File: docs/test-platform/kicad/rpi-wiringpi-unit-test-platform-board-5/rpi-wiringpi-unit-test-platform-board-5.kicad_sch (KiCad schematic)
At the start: 14 parts, among them J1 JST_IN_PWR, J2 JST_IN_SIG, J3 JST_IN_LCD, J4 JST_OUT_ARDUINO, M1 Logic_Converter_4_Pin, SW1 SW_CTRL

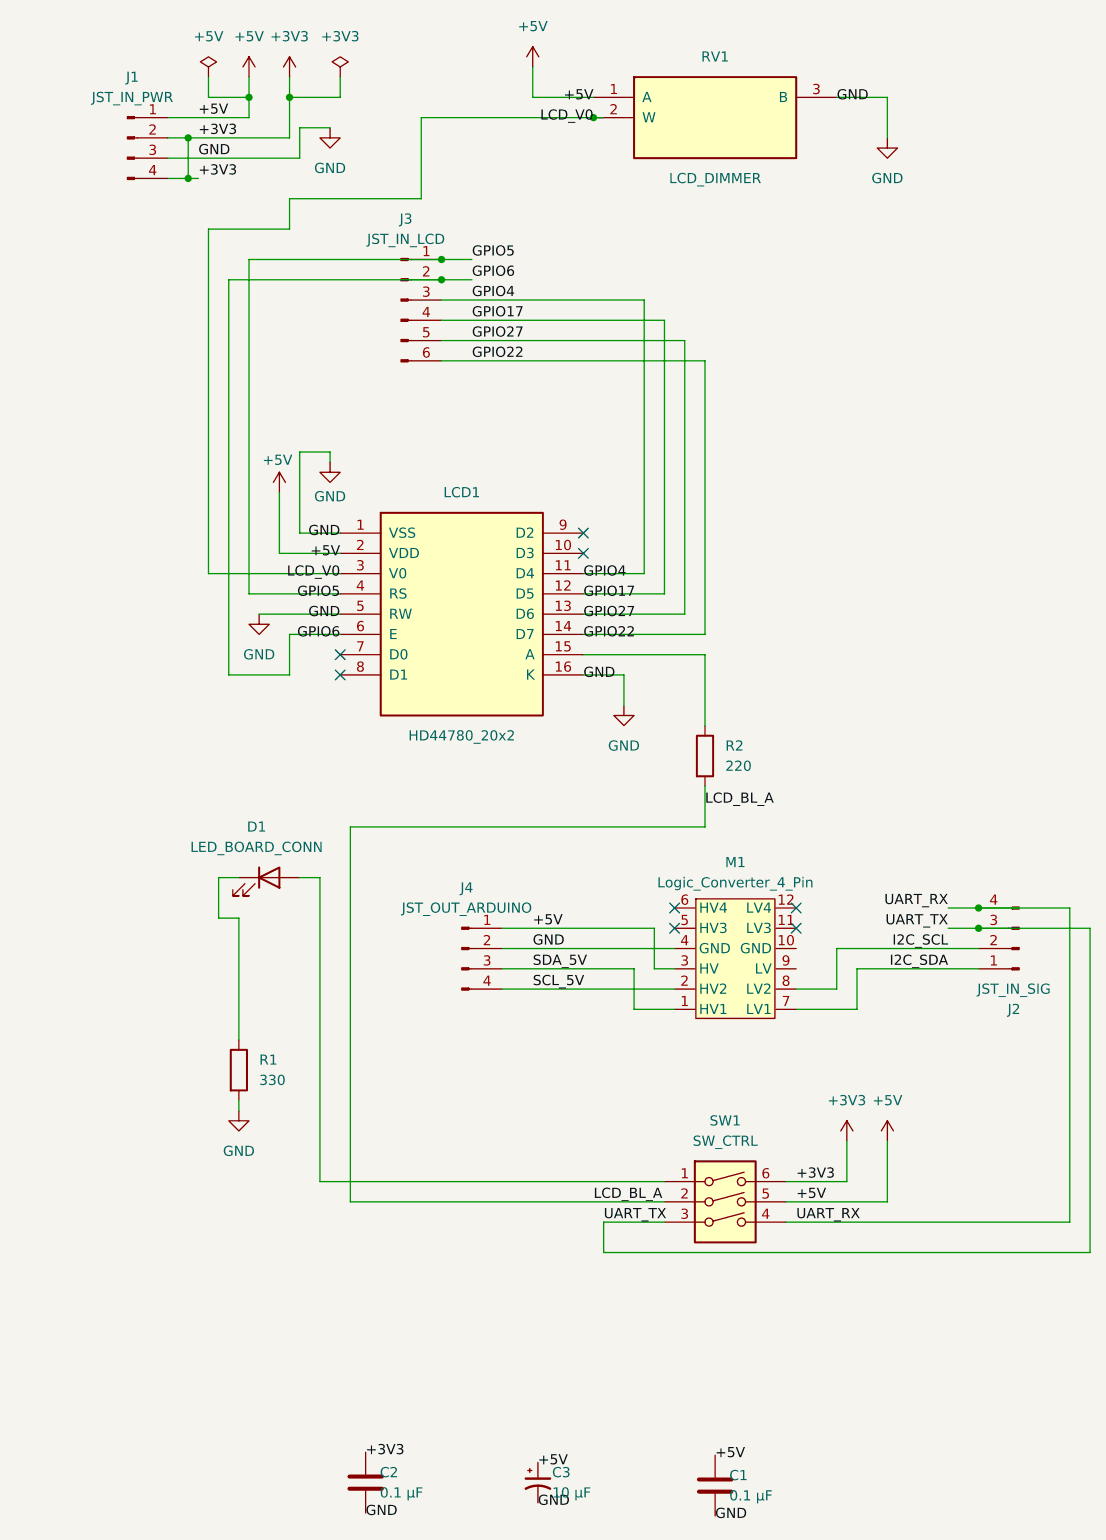
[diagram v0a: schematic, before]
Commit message: Finished test board 5
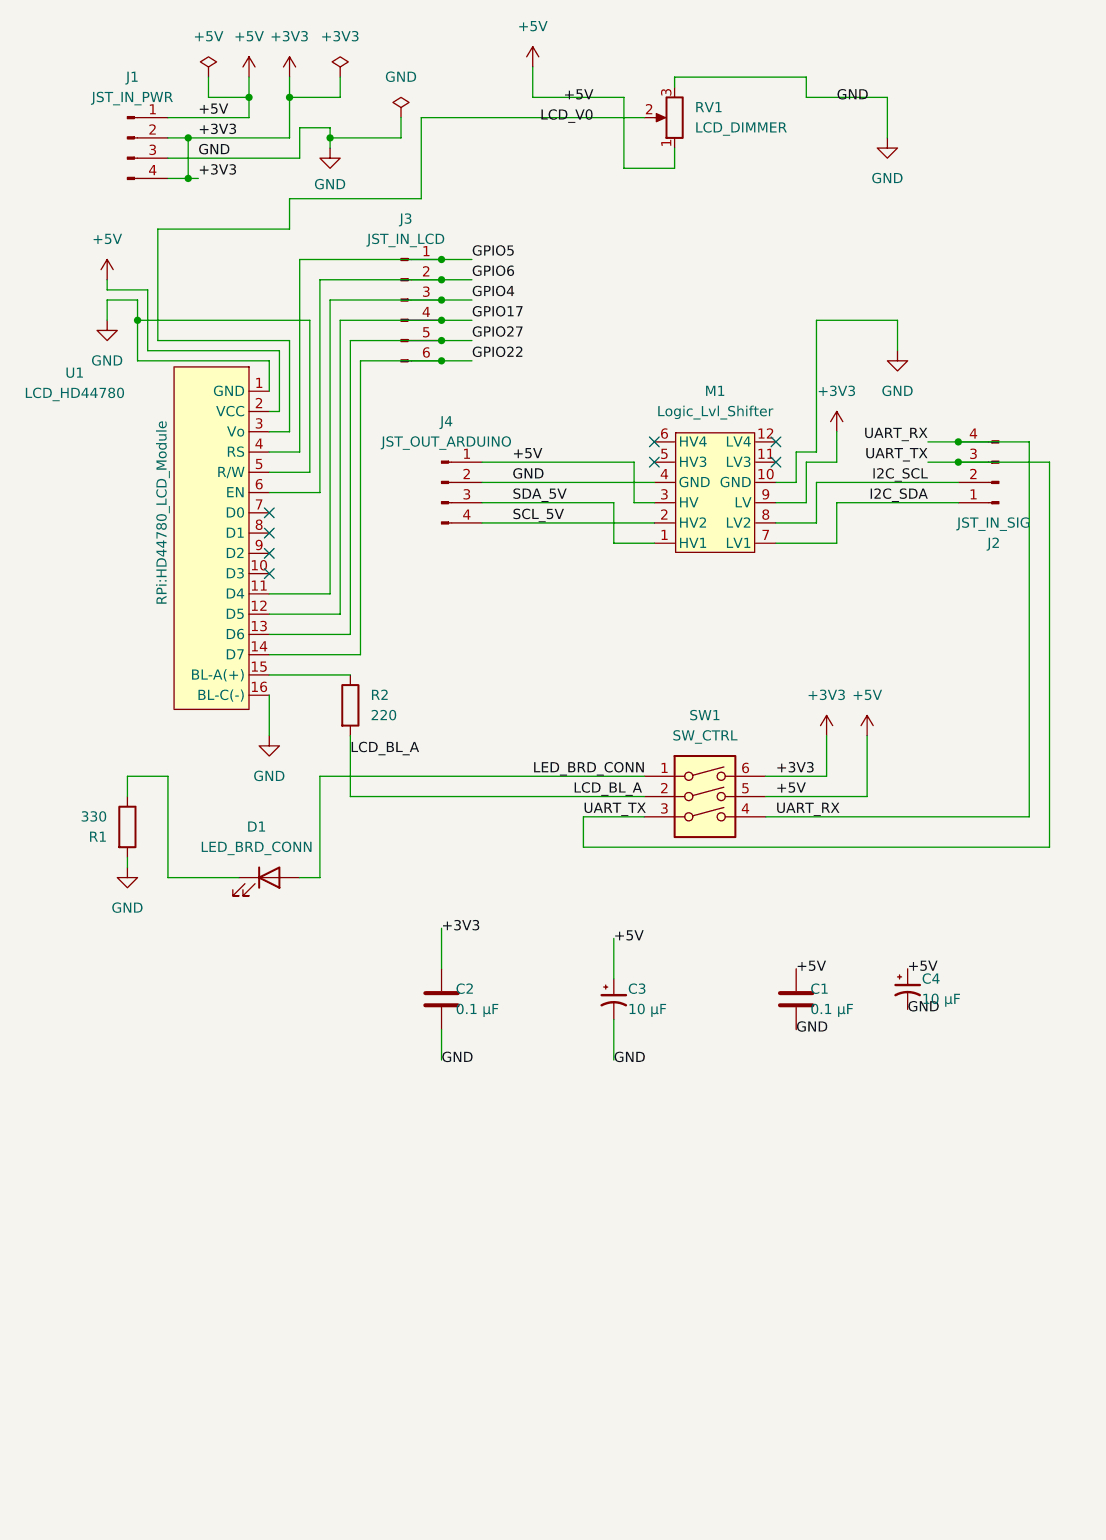
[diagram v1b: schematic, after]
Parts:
- removed LCD1: HD44780_20x2, RPi:HD44780_LCD_Module, symbol rpi-wiringpi-unit-test-platform-board-5:LCD1
- removed RV1: LCD_DIMMER, Potentiometer_THT:Potentiometer_Alps_RK09K_Single_Vertical, symbol rpi-wiringpi-unit-test-platform-board-5:RV1
- added C4: 10 µF, Capacitor_THT:CP_Radial_D5.0mm_P2.50mm, symbol Device:C_Polarized_Small_US
- added RV1: LCD_DIMMER, Potentiometer_THT:Potentiometer_Alps_RK09K_Single_Vertical, symbol Device:R_Potentiometer
- added U1: LCD_HD44780, RPi:HD44780_LCD_Module, symbol RPi:LCD_HD44780
- D1: value LED_BOARD_CONN -> LED_BRD_CONN
- M1: value Logic_Converter_4_Pin -> Logic_Lvl_Shifter
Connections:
- net +3V3: now also M1.9 (LV)
- net +5V: now also C4.1, RV1.1, U1.2 (VCC)
- net GND: now also M1.10 (GND), C4.2, RV1.3, U1.1 (GND), U1.16 (BL-C(-)), U1.5 (R/W)
- net GPIO17: now also U1.12 (D5)
- net GPIO22: now also U1.14 (D7)
- net GPIO27: now also U1.13 (D6)
- net GPIO4: now also U1.11 (D4)
- net GPIO5: now also U1.4 (RS)
- net GPIO6: now also U1.6 (EN)
- net LCD_V0: now also RV1.2, U1.3 (Vo)
- net at R2.1: now also U1.15 (BL-A(+))
- net LED_BRD_CONN: now reaches D1.2 (A), SW1.1
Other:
- moved on the sheet: C1, C2, C3, J2, J4, M1, R1, R2, SW1
